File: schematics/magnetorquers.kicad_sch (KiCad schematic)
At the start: 12 parts, among them U10 DRV8837C, U3 DRV8837C, U4 DRV8837C

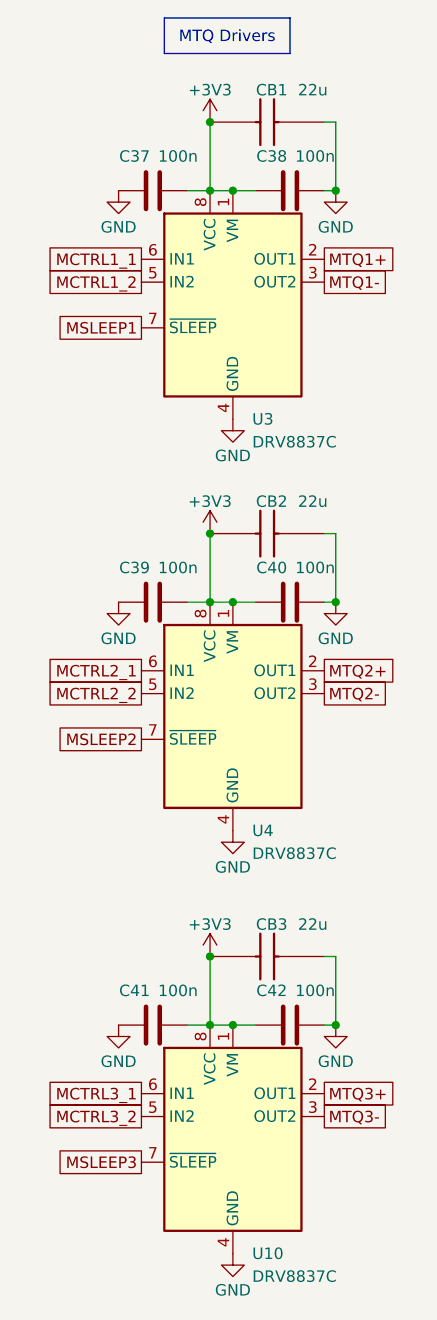
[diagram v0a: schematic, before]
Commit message: fix BOM, generate .pos, fix component values, re-plot schematics
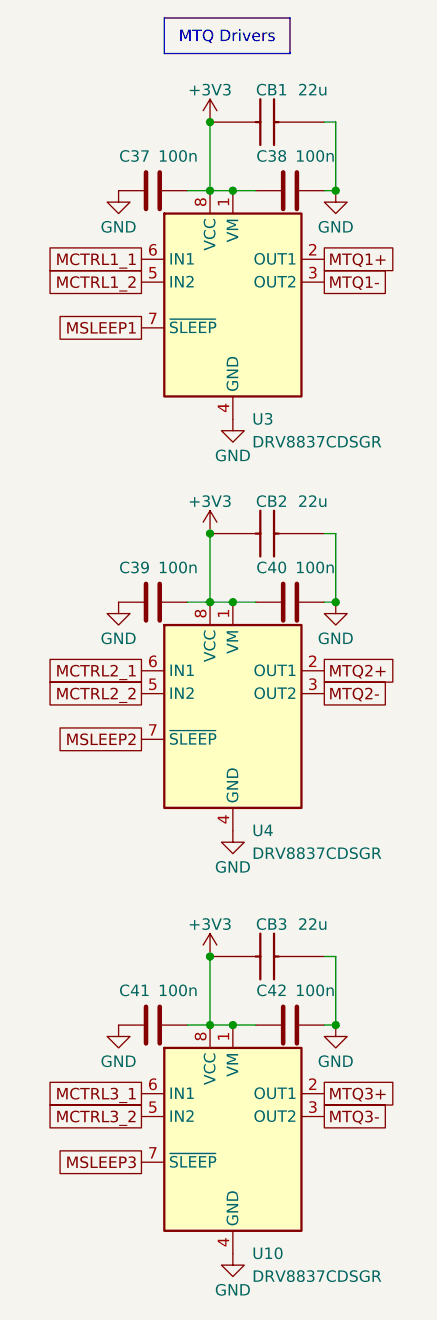
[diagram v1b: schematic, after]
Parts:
- U10, U3, U4: value DRV8837C -> DRV8837CDSGR; Manufacturer_Name (none) -> Texas Instruments; Manufacturer_Part_Number (none) -> DRV8837CDSGR
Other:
- company: (none) -> Brown Space Engineering
- title: (none) -> PVDX ADCS/PMB
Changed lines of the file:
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@@
 	(generator_version "10.0")
 	(paper "A4")
+	(title_block
+		(title "PVDX ADCS/PMB")
+		(date "2026-09-04")
+		(rev "1.1")
+		(company "Brown Space Engineering")
+	)
 	(text_box "MTQ Drivers"
 		(exclude_from_sim no)
@@
 			)
 		)
-		(property "Value" "DRV8837C"
+		(property "Value" "DRV8837CDSGR"
 			(at 116.4433 128.27 0)
 			(show_name no)
@@
 		)
 		(property "Description" "H-Bridge driver, 1A, Low Voltage, PWM input, WSON-8"
+			(at 114.3 113.03 0)
+			(hide yes)
+			(show_name no)
+			(do_not_autoplace no)
+			(effects
+				(font
+					(size 1.27 1.27)
+				)
+			)
+		)
+		(property "Manufacturer_Name" "Texas Instruments"
+			(at 114.3 113.03 0)
+			(hide yes)
+			(show_name no)
+			(do_not_autoplace no)
+			(effects
+				(font
+					(size 1.27 1.27)
+				)
+			)
+		)
+		(property "Manufacturer_Part_Number" "DRV8837CDSGR"
 			(at 114.3 113.03 0)
 			(hide yes)
@@
 			)
 		)
-		(property "Value" "DRV8837C"
+		(property "Value" "DRV8837CDSGR"
 			(at 116.4433 175.26 0)
 			(show_name no)
@@
 		)
 		(property "Description" "H-Bridge driver, 1A, Low Voltage, PWM input, WSON-8"
+			(at 114.3 160.02 0)
+			(hide yes)
+			(show_name no)
+			(do_not_autoplace no)
+			(effects
+				(font
+					(size 1.27 1.27)
+				)
+			)
+		)
+		(property "Manufacturer_Name" "Texas Instruments"
+			(at 114.3 160.02 0)
+			(hide yes)
+			(show_name no)
+			(do_not_autoplace no)
+			(effects
+				(font
+					(size 1.27 1.27)
+				)
+			)
+		)
+		(property "Manufacturer_Part_Number" "DRV8837CDSGR"
 			(at 114.3 160.02 0)
 			(hide yes)
@@
 			)
 		)
-		(property "Value" "DRV8837C"
+		(property "Value" "DRV8837CDSGR"
 			(at 116.4433 82.55 0)
 			(show_name no)
@@
 			(at 114.3 67.31 0)
 			(hide yes)
+			(show_name no)
+			(do_not_autoplace no)
+			(effects
+				(font
+					(size 1.27 1.27)
+				)
+			)
+		)
+		(property "Manufacturer_Name" "Texas Instruments"
+			(at 114.3 67.31 0)
+			(hide yes)
+			(show_name no)
+			(do_not_autoplace no)
+			(effects
+				(font
+					(size 1.27 1.27)
+				)
+			)
+		)
+		(property "Manufacturer_Part_Number" "DRV8837CDSGR"
+			(at 114.3 67.31 0)
+			(hide yes)
